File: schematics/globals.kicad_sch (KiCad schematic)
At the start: 28 parts, among them J1 Power, U11 74HC590, U17 ATF22V10C-7, U2 74HCU04, U20 74HC590, U21 74HC590, U22 SST39SF010A-70-4C-PHE, U7 74HC14, Y3 12MHz

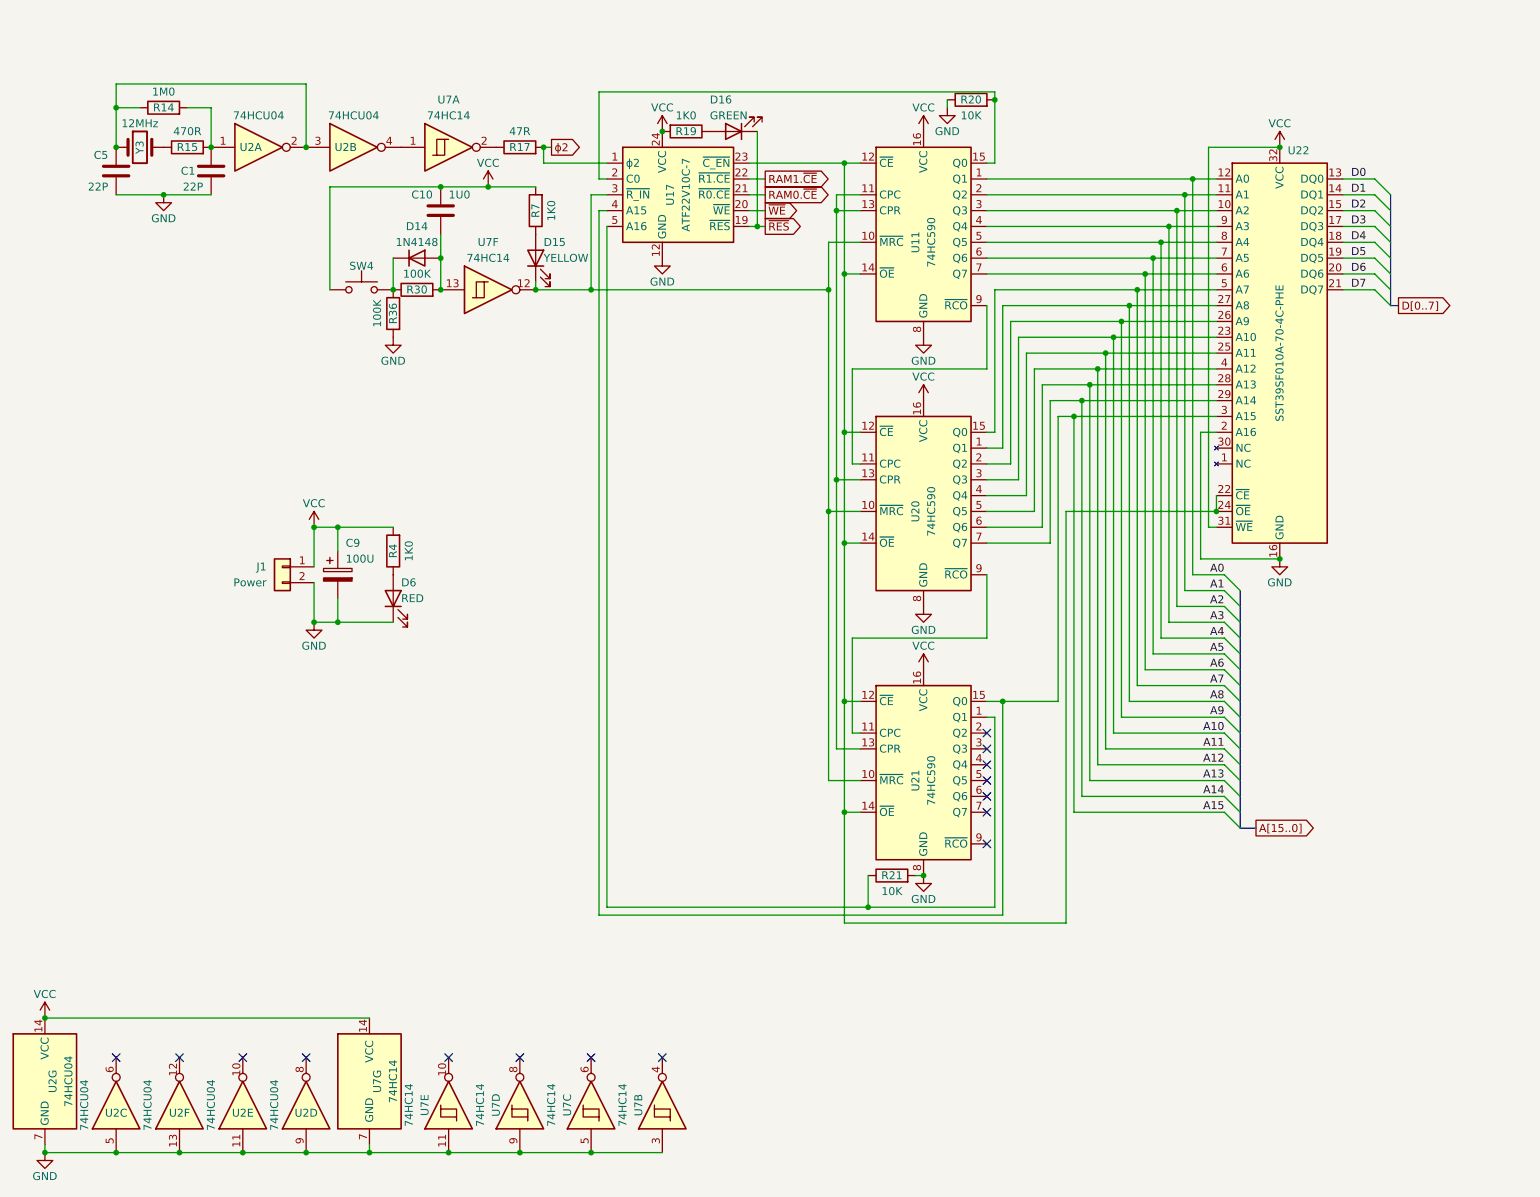
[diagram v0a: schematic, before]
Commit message: added phi0 for write latch timing
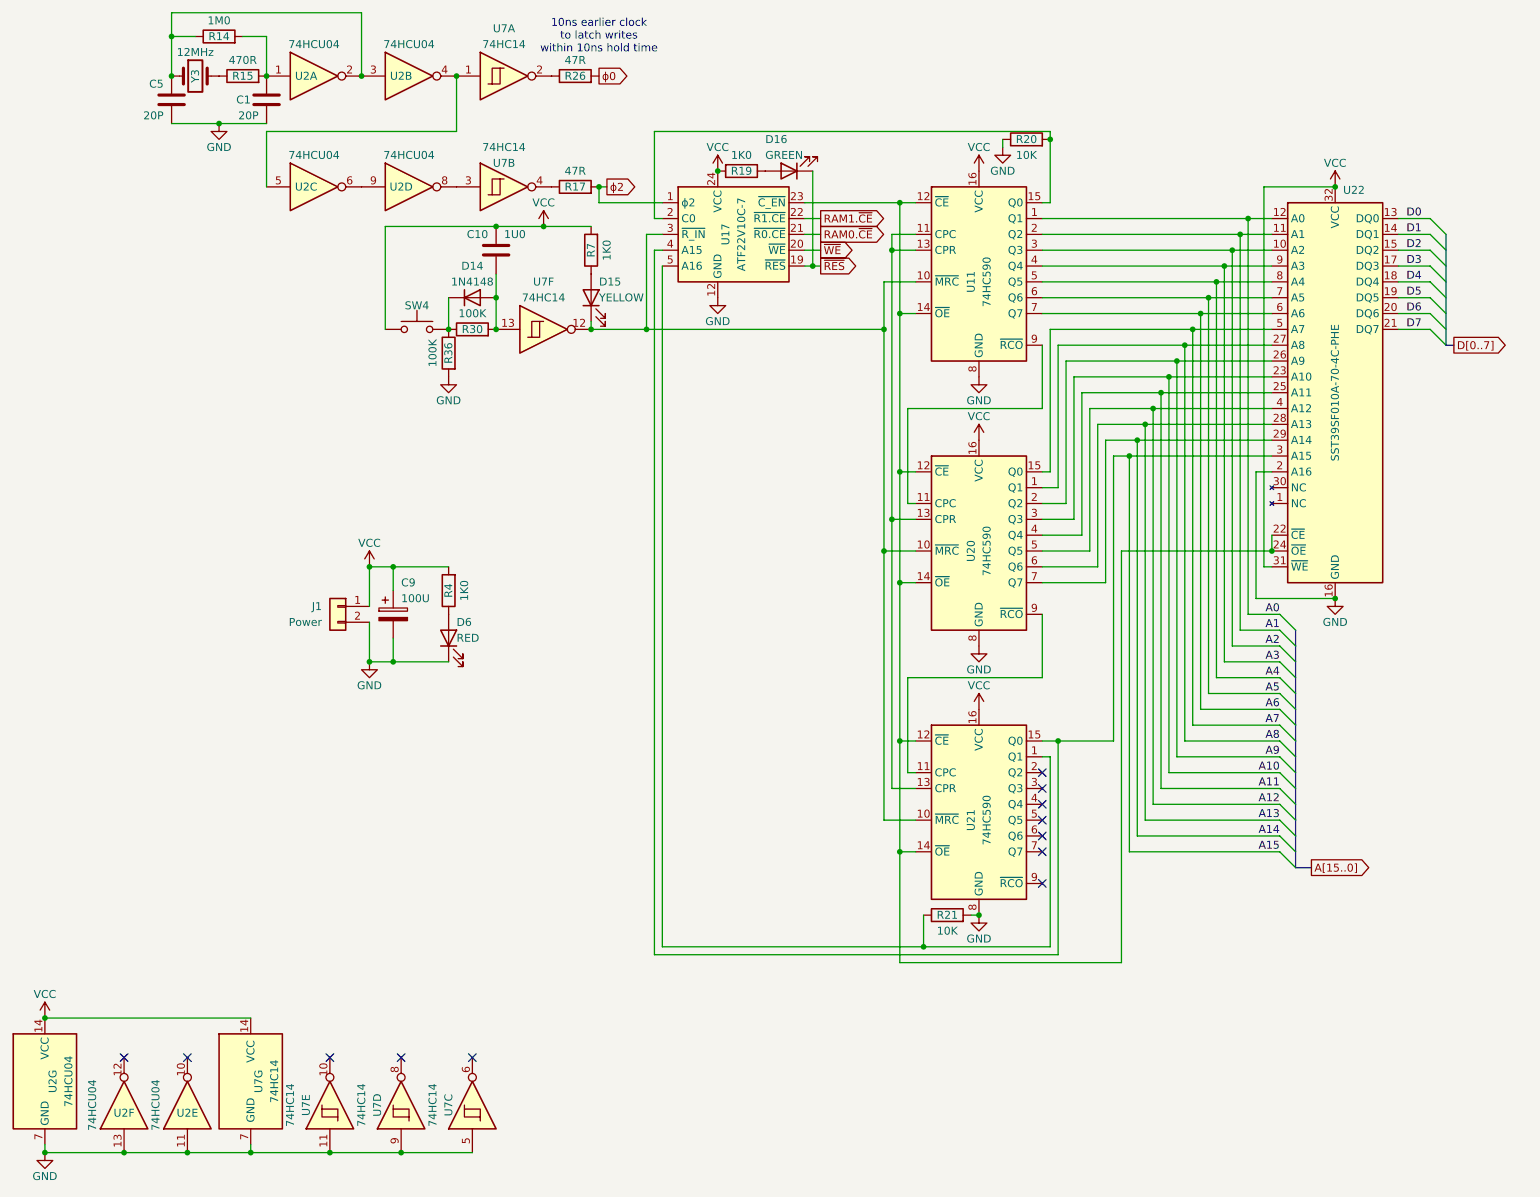
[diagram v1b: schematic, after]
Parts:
- added R26: 47R, symbol Device:R
- C1, C5: value 22P -> 20P
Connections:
- net GND: no longer U2.5, U2.9, U7.3
- net at U2.8: now also U7.3
- net at U2.4, U7.1: now also U2.5
- net at U2.6: now also U2.9
- net at U7.2: now also R26.1; no longer R17.1
- net at U7.4: now also R17.1
- new net ϕ0: R26.2
- no-connect marks 15 -> 12
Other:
- note added: "10ns earlier clock to latch writes within 10ns hold time"
- moved on the sheet: C1, C10, C5, C9, D14, D15, D16, D6, J1, R14, R15, R17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
